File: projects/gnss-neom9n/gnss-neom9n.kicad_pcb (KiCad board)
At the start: 2 copper layers, 34 x 40 mm, 27 parts, among them J1 PWR-IN, J2 U.FL-ANT, J3 UART-I2C, J4 PPS-INT, SW1 RESET, U1 XC6206P332MR, U2 NEO-M9N-00B

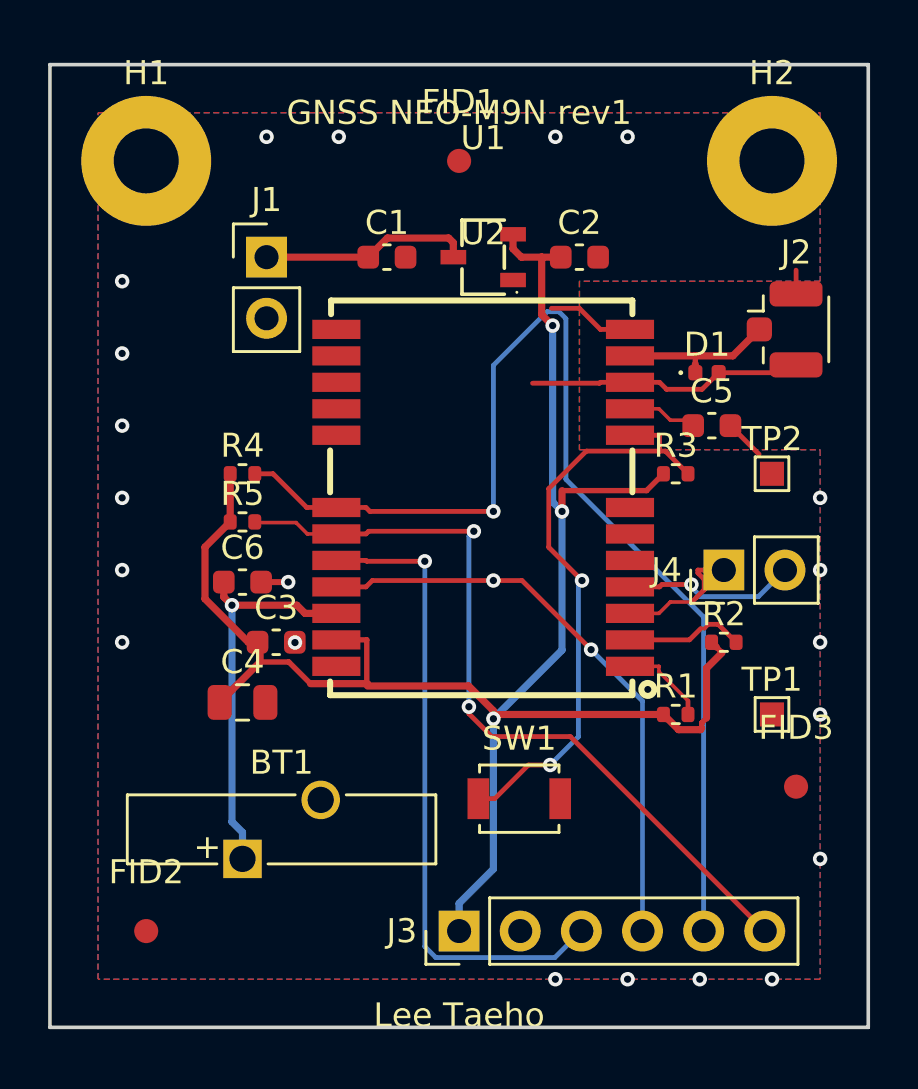
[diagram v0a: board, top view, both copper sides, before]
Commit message: 9/6 update
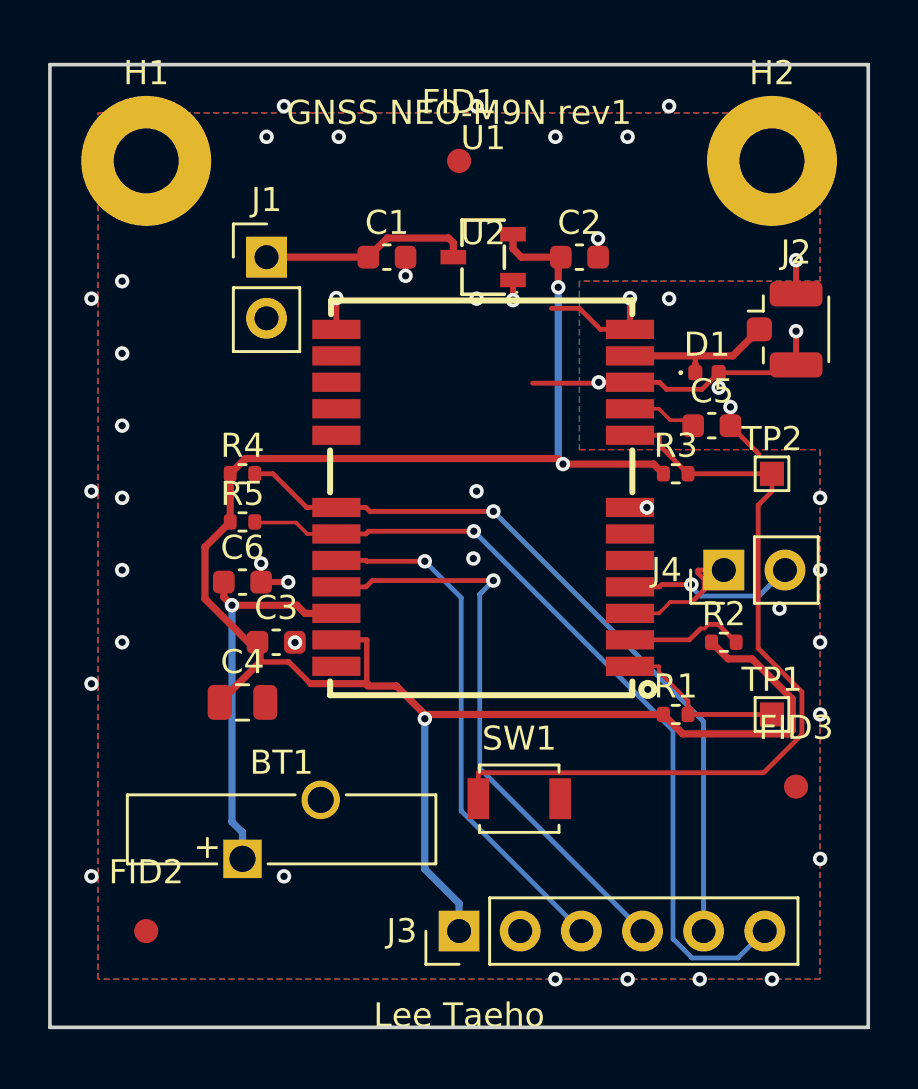
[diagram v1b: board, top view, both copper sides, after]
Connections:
- TP1 pad 1: (no net) -> SAFEBOOT_N
- TP2 pad 1: (no net) -> RESET_N
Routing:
- net I2C_SDA: track 48.5 -> 31.6 mm
- net GND: track 18.9 -> 30.9 mm, vias 21 -> 46
- net RESET_N: track 24.9 -> 33.8 mm, vias 2 -> 0
- net VCC: track 77.1 -> 83.5 mm
- net UART_TXD: track 26.8 -> 21.7 mm
- net SAFEBOOT_N: track 3.70 -> 7.19 mm
- net I2C_SCL: track 33.1 -> 34.3 mm, vias 2 -> 1
- net UART_RXD: track 24.5 -> 24.2 mm, vias 2 -> 1
